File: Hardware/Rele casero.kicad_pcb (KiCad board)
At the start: 2 copper layers, 15 parts, among them J1 Screw_Terminal_01x02, J2 Screw_Terminal_01x02, K1 SANYOU_SRD_Form_C, Q1 PN2222A, U1 ESP32C3-SUPERMINI, U2 4N25, U4 SMTS-102

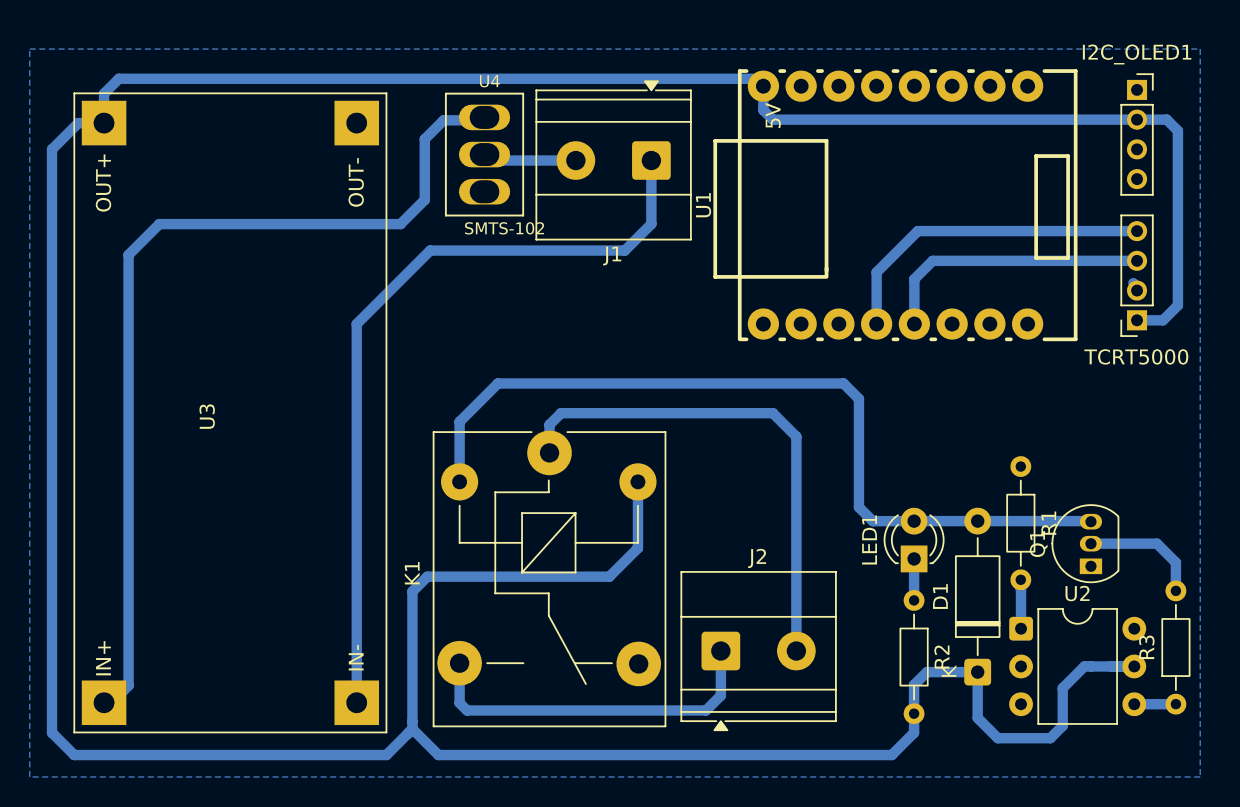
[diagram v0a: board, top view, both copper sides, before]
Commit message: Add files via upload
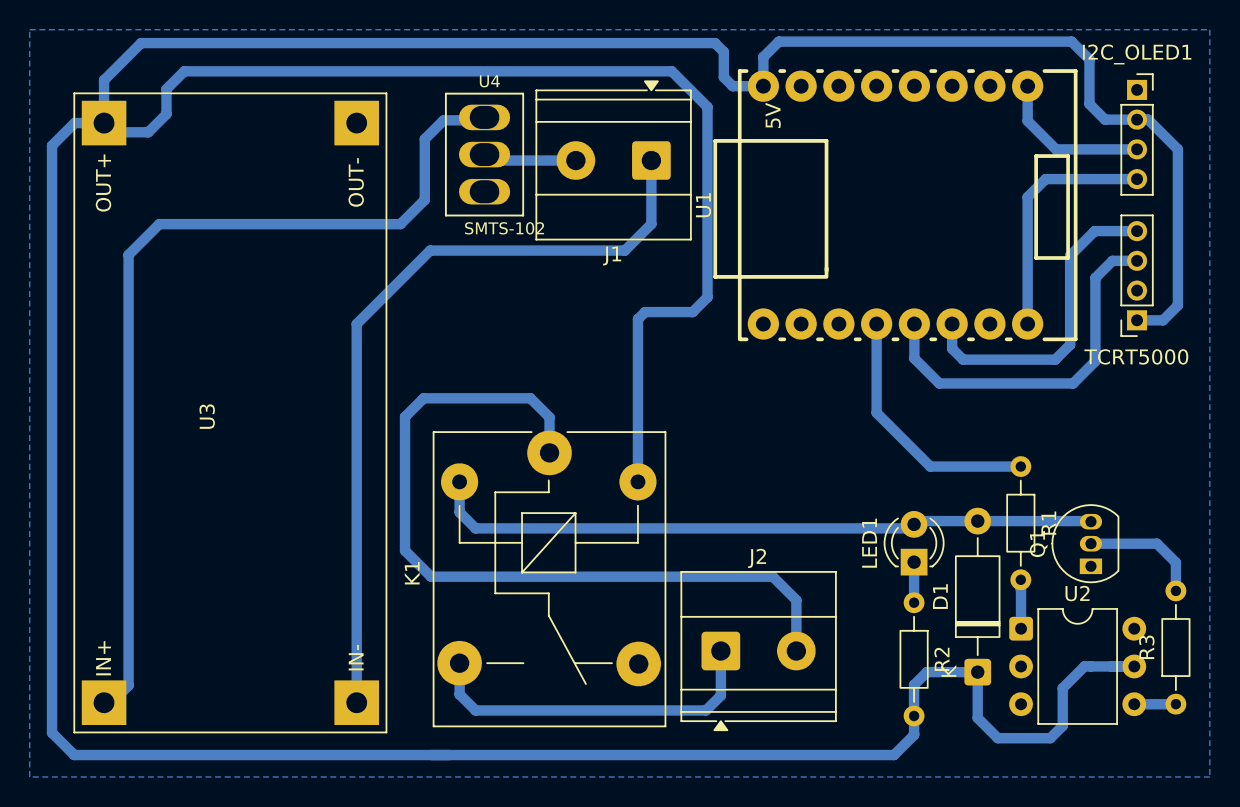
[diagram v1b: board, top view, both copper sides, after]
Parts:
- moved LED1 0.21 mm to (101.5, 104.0)
- moved R2 0.15 mm to (101.5, 106.8)
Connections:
- U1 pad 4: A0 -> Micro
- U1 pad 6: unconnected-(U1-GPIO10-Pad6) -> A0
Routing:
- net VCC: track 254.9 -> 304.5 mm
- net Net-(J2-Pin_2): track 33.9 -> 53.3 mm
- net Micro: track 0.00 -> 17.2 mm
- net SDA: track 0.00 -> 16.4 mm
- net Net-(D1-A): track 55.7 -> 44.6 mm
- net SCL: track 0.00 -> 10.5 mm
- net D0: track 18.5 -> 24.7 mm
- net A0: track 22.1 -> 21.5 mm
